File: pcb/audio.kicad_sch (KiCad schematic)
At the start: 56 parts, among them Q10 BC547, Q7 BC547, Q8 BC547, Q9 BC547, U58 LM7809_TO220, U59 LM7805_TO220, U60 LM7909_TO220, U61 74HC245, U62 4504, U63 4053, U64 4053, U65 4504, U66 4053, U67 TL072, U68 4053

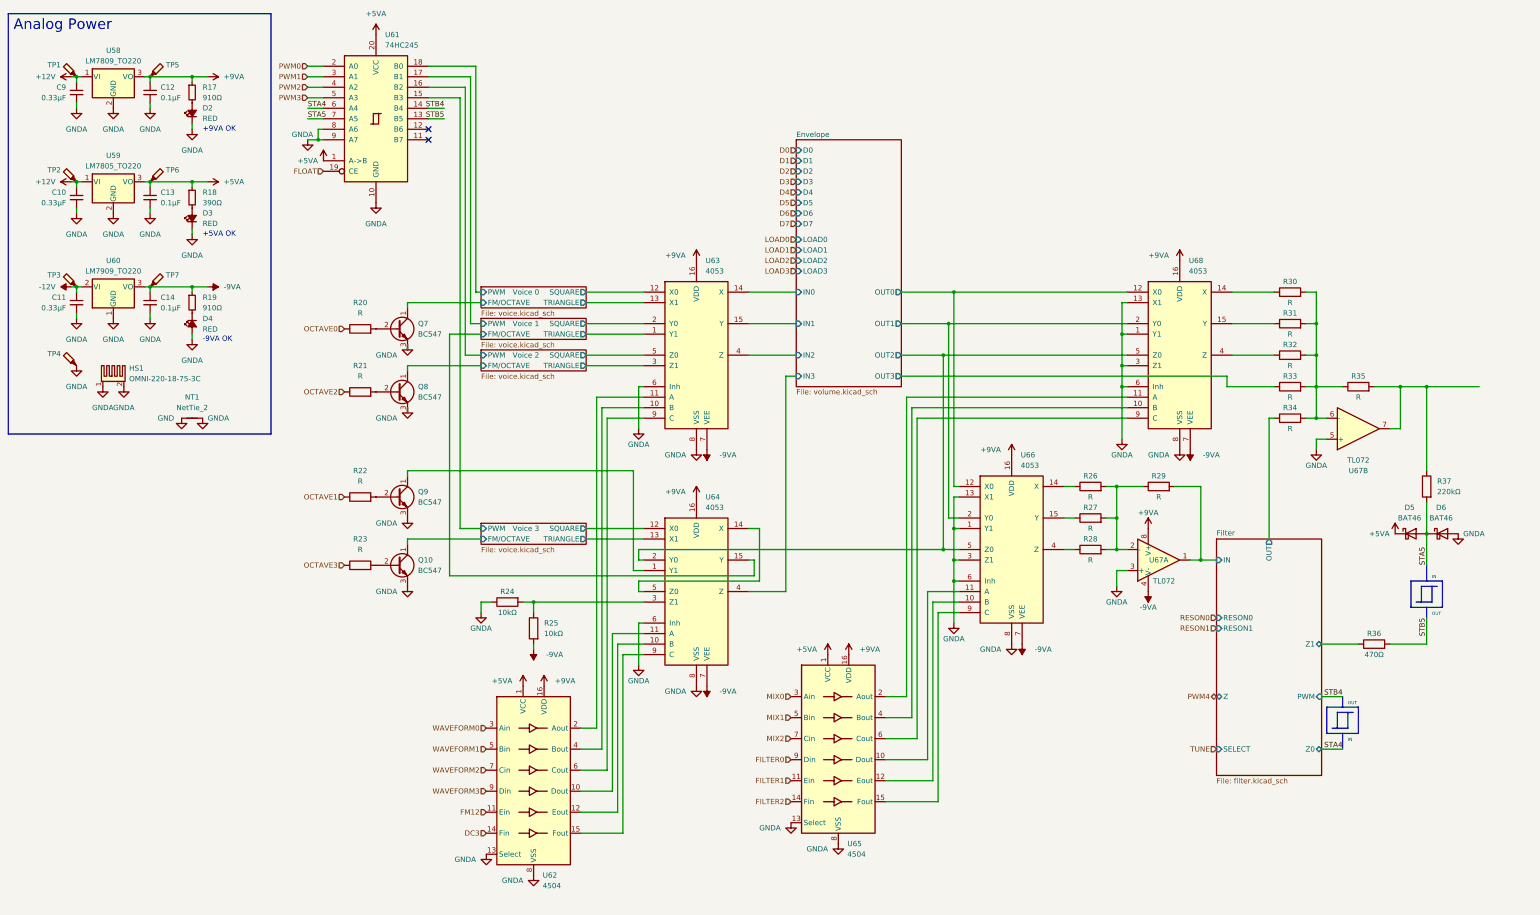
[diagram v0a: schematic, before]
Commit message: WIP schematic
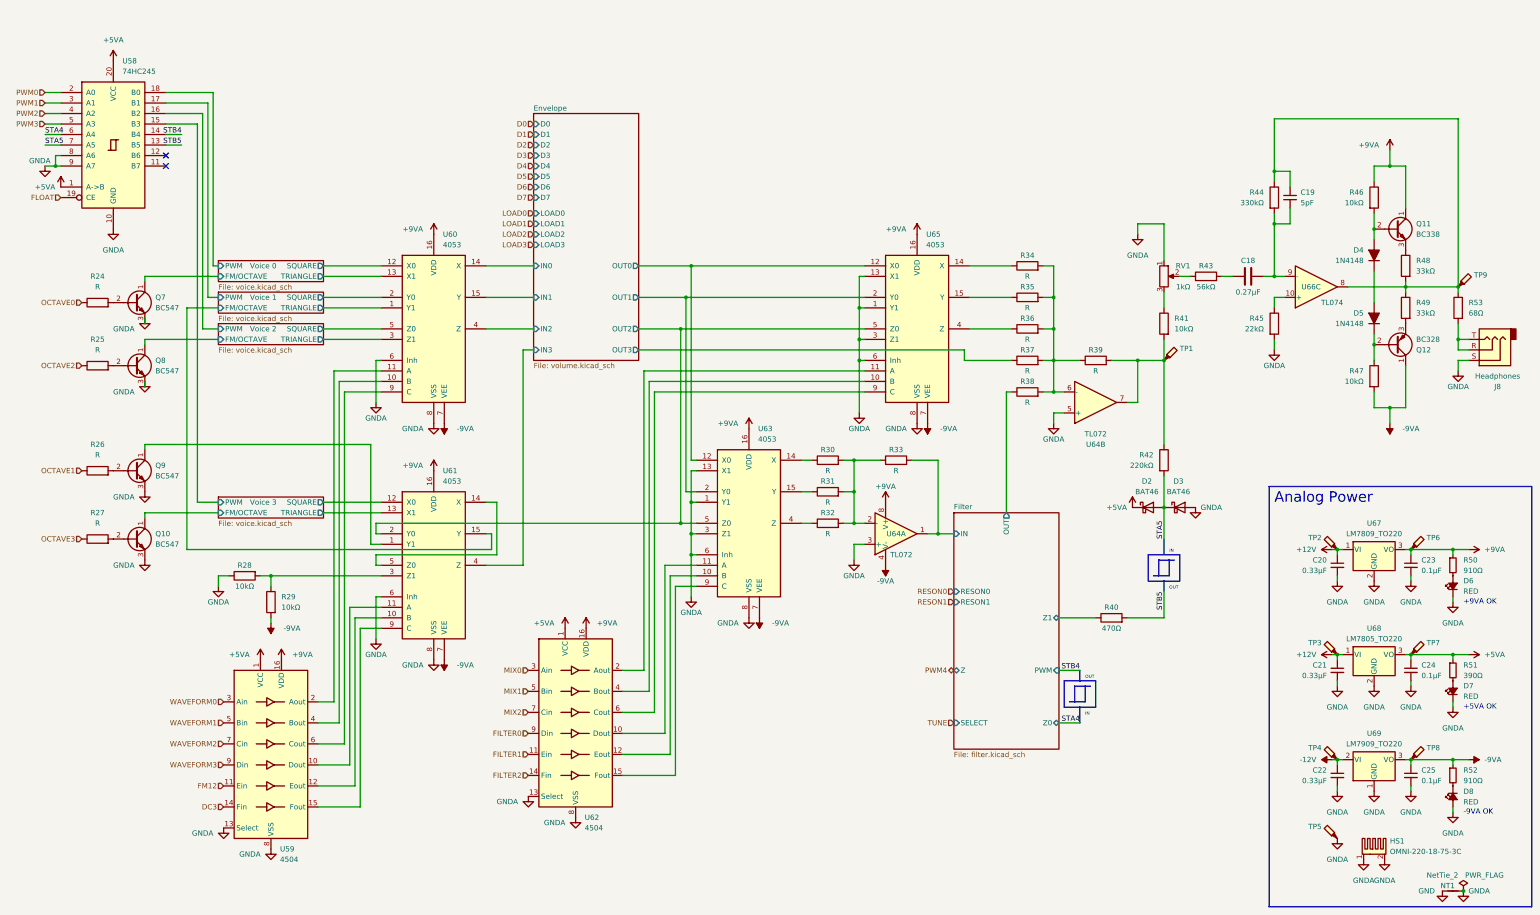
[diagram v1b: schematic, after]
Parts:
- added C18: 0.27µF, symbol Device:C
- added C19: 5pF, symbol Device:C_Small
- added D4, D5: 1N4148, symbol Device:D_Filled
- added J8: Headphones, symbol Connector_Audio:AudioJack3
- added Q11: BC338, Package_TO_SOT_THT:TO-92_Inline, symbol Transistor_BJT:BC338
- added Q12: BC328, Package_TO_SOT_THT:TO-92_Inline, symbol Transistor_BJT:BC328
- added R41, R46, R47: 10kΩ, symbol Device:R
- added R43: 56kΩ, symbol Device:R
- added R44: 330kΩ, symbol Device:R
- added R45: 22kΩ, symbol Device:R
- added R48, R49: 33kΩ, symbol Device:R
- added R53: 68Ω, symbol Device:R
- added RV1: 1kΩ, symbol Device:R_Potentiometer
- added TP1, TP9: TestPoint_Probe, symbol Connector:TestPoint_Probe
- added U66: TL074, symbol Amplifier_Operational:TL074
- renumbered C9 to C20, C10 to C21, C11 to C22, C12 to C23, C13 to C24, C14 to C25, D5 to D2, D6 to D3, D2 to D6, D3 to D7, D4 to D8, R20 to R24, R21 to R25, R22 to R26, R23 to R27, R24 to R28, R25 to R29, R26 to R30, R27 to R31, R28 to R32, R29 to R33, R30 to R34, R31 to R35, R32 to R36, R33 to R37, R34 to R38, R35 to R39, R36 to R40, R37 to R42, R17 to R50, R18 to R51, R19 to R52, TP1 to TP2, TP2 to TP3, TP3 to TP4, TP4 to TP5, TP5 to TP6, TP6 to TP7, TP7 to TP8, U61 to U58, U62 to U59, U63 to U60, U64 to U61, U65 to U62, U66 to U63, U67 to U64, U68 to U65, U58 to U67, U59 to U68, U60 to U69
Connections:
- net +9VA: now also Q11.1 (C), R46.1
- net -9VA: now also Q12.1 (C), R47.2
- net GNDA: now also J8.S, R45.2, RV1.1
- net at R39.2, R42.1, U64.7: now also R41.2, TP1.1
- new net: R43.1, RV1.2
- new net: R41.1, RV1.3
- new net: J8.R, J8.T, R53.2
- new net: C19.1, R44.1, R48.2, R49.1, R53.1, TP9.1, U66.8
- new net: C18.2, C19.2, R44.2, U66.9 (-)
- new net: Q11.3 (E), R48.1
- new net: D4.2 (A), Q11.2 (B), R46.2
- new net: D5.1 (K), Q12.2 (B), R47.1
- new net: D4.1 (K), D5.2 (A)
- new net: Q12.3 (E), R49.2
- new net: R45.1, U66.10 (+)
- new net: C18.1, R43.2
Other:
- moved on the sheet: C20, C21, C22, C23, C24, C25, D2, D3, D6, D7, D8, HS1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
